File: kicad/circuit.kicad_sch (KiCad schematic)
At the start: 20 parts, among them SW1 {dblquote}Snap wire{dblquote}, U1 RaspberryPi_Pico, U2 74HC595

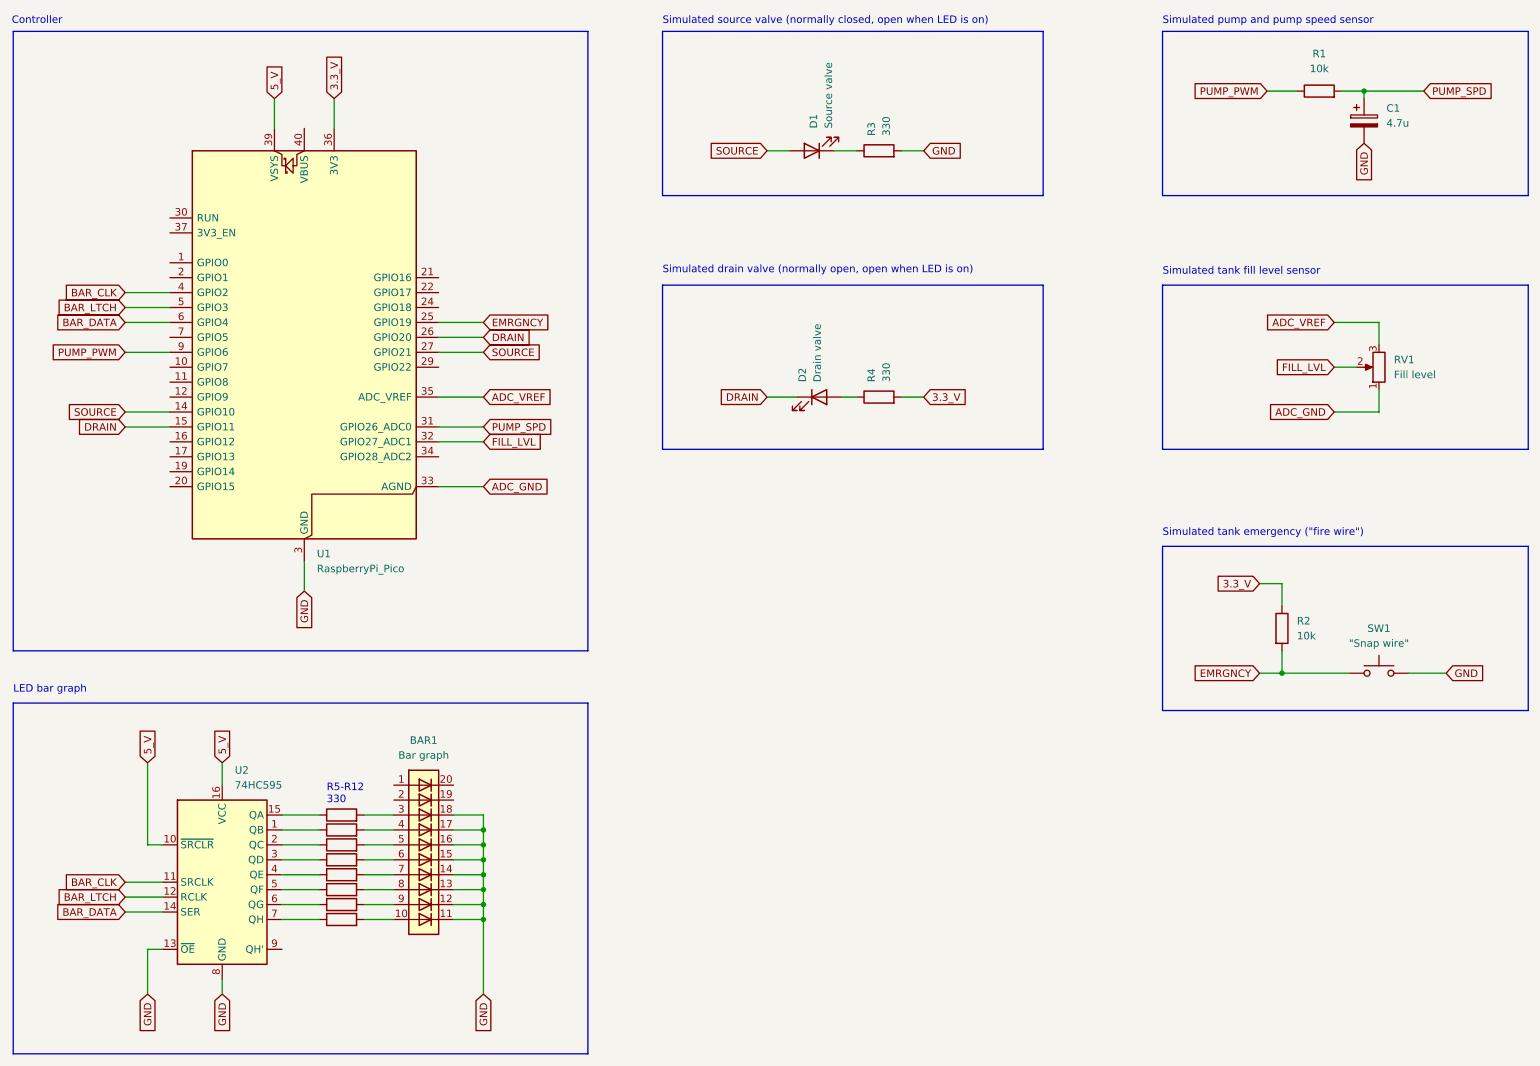
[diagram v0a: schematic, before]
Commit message: Update schematic and diagram.
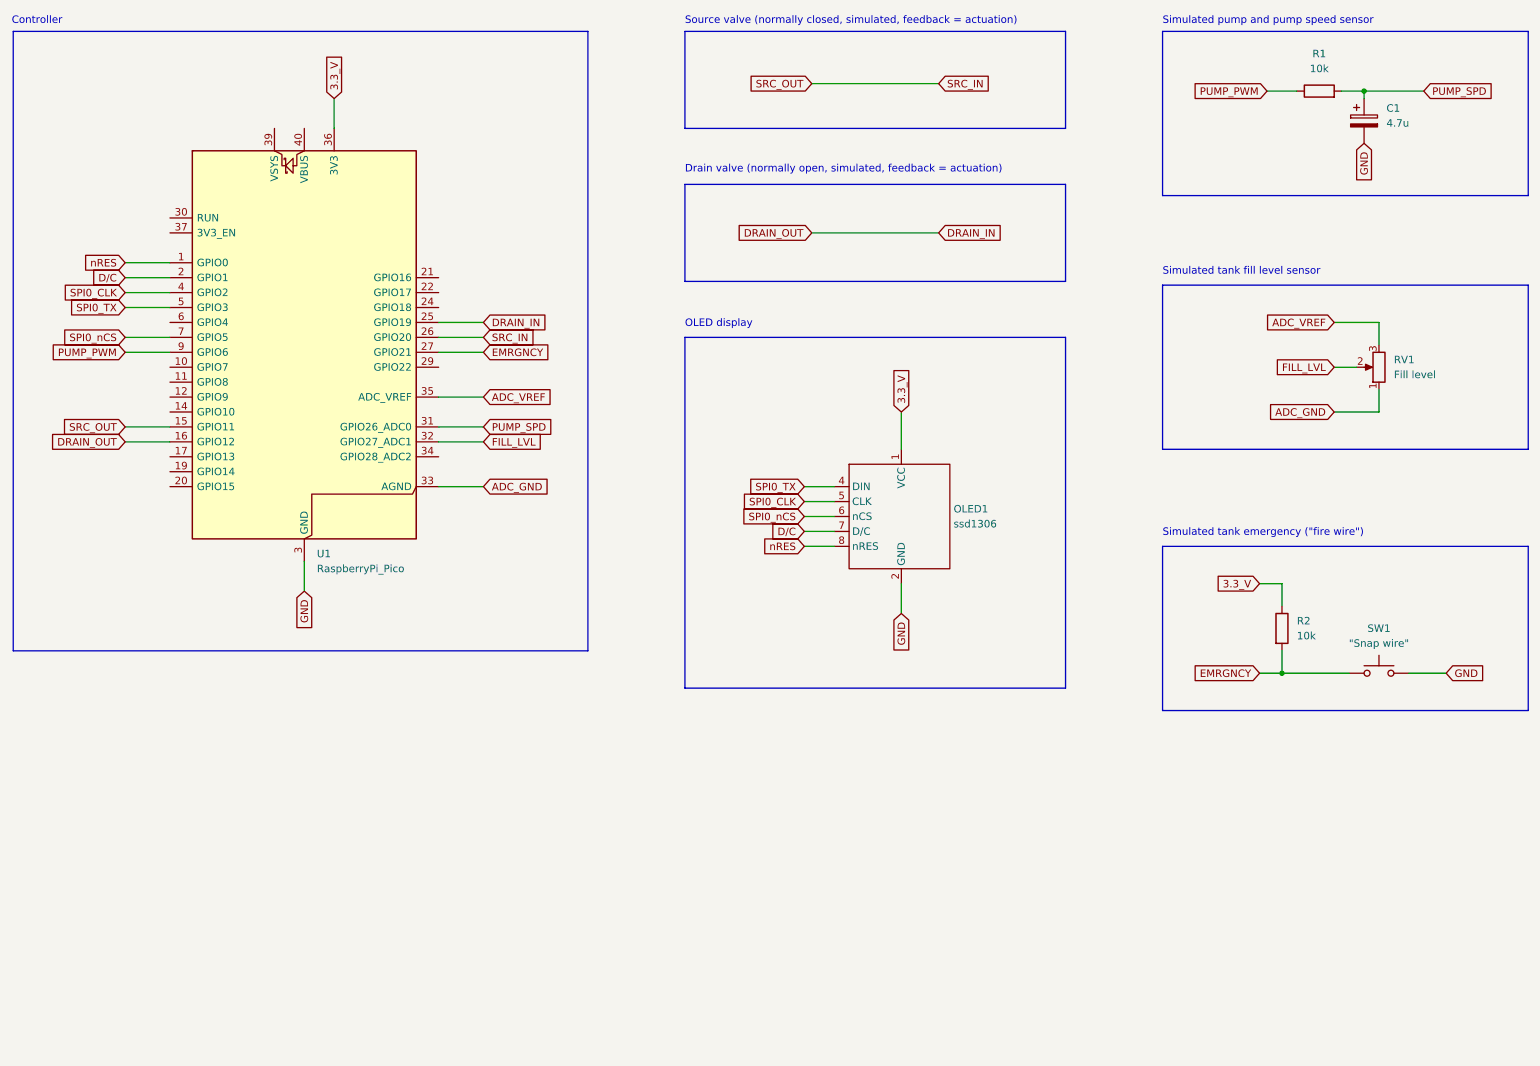
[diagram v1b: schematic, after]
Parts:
- removed BAR1: Bar graph, Display:HDSP-4830, symbol LED:HDSP-4830_2
- removed D1: Source valve, symbol Device:LED
- removed D2: Drain valve, symbol Device:LED
- removed R10, R11, R12, R3, R4, R5, R6, R7, R8, R9: 330, symbol Device:R
- removed U2: 74HC595, symbol 74xx:74HC595
- added OLED1: ssd1306, symbol pico-rio:ssd1306
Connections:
- net 3.3_V: now also OLED1.1 (VCC)
- net EMRGNCY: now also U1.27 (GPIO21); no longer U1.25 (GPIO19)
- net GND: now also OLED1.2 (GND)
- net nRES: now reaches U1.1 (GPIO0)
- net nRES: now also OLED1.8 (nRES)
- net DRAIN_IN: now reaches U1.16 (GPIO12)
- net DRAIN_IN: now also U1.25 (GPIO19)
- net D/C: now reaches U1.2 (GPIO1)
- net D/C: now also OLED1.7 (D/C)
- net SPI0_nCS: now reaches U1.7 (GPIO5)
- net SPI0_nCS: now also OLED1.6 (nCS)
- net 5_V: no longer names the net of U1.39 (VSYS)
- net BAR_CLK renamed SPI0_CLK
- net SPI0_CLK: now also OLED1.5 (CLK)
- net BAR_DATA: no longer names the net of U1.6 (GPIO4)
- net BAR_LTCH renamed SPI0_TX
- net SPI0_TX: now also OLED1.4 (DIN)
- net DRAIN renamed SRC_IN
- net SOURCE: no longer names the net of U1.14 (GPIO10)
- net SOURCE: no longer U1.27 (GPIO21)
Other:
- note added: "Drain valve (normally open, simulated, feedback = actuation)"
- note added: "OLED display"
- note added: "Source valve (normally closed, simulated, feedback = actuation)"
- note removed: "LED bar graph"
- note removed: "R5-R12 330"
- note removed: "Simulated drain valve (normally open, open when LED is on)"
- note removed: "Simulated source valve (normally closed, open when LED is on)"
